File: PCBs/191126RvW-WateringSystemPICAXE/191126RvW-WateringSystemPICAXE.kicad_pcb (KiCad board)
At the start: 2 copper layers, 83.8 x 38.1 mm, 17 parts, among them J1 MotorConn, J2 SerIn, J3 SerSelect, J4 SerOut, J5 Screw_Terminal_01x04, J6 SerSelect, Q1 KN2222A, U1 PICAXEM2

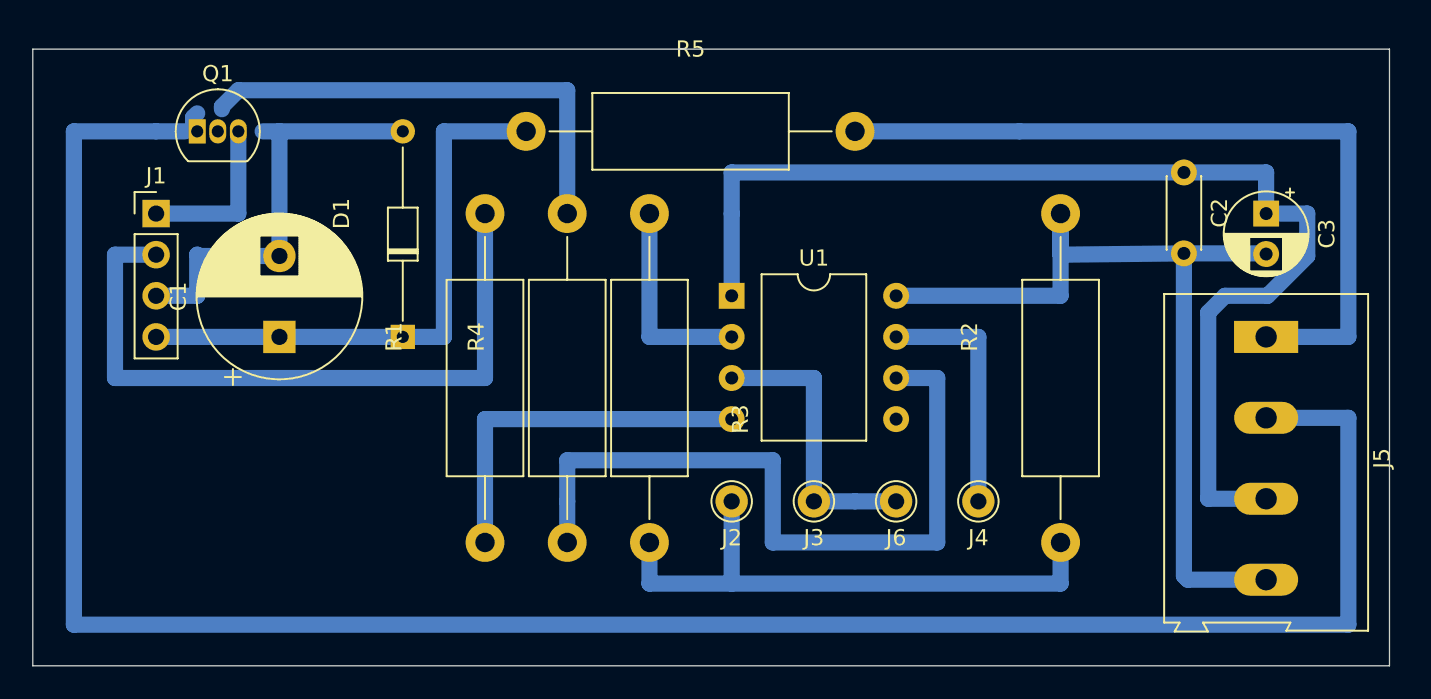
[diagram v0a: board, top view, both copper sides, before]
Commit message: pcb changes
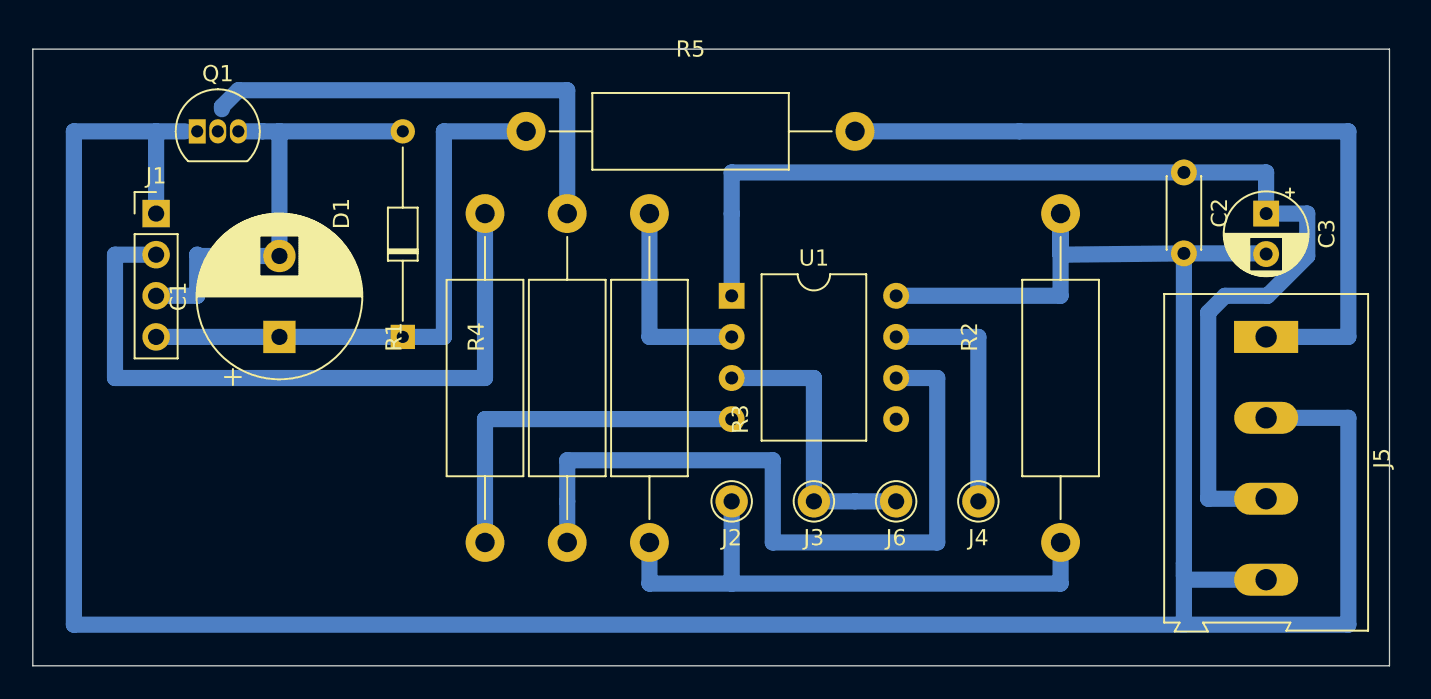
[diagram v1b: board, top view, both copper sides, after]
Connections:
- J1 pad 1: GNDPWR -> GNDD
- J5 pad 2: GNDPWR -> GNDD
- Q1 pad 1: GNDPWR -> GNDD
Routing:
- net GNDPWR: track 145.3 -> 0.00 mm
- net GNDD: track 55.5 -> 198.3 mm
- net Net-(C1-Pad2): track 26.6 -> 27.8 mm
